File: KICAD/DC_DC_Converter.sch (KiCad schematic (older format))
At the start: 5 parts

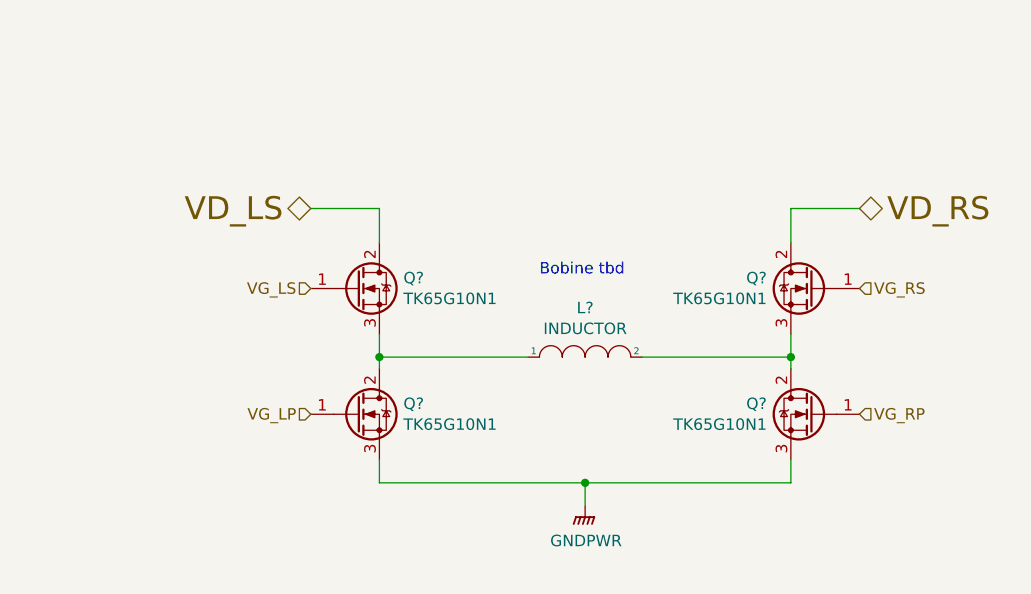
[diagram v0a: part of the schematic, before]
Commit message: ebauche driver mos
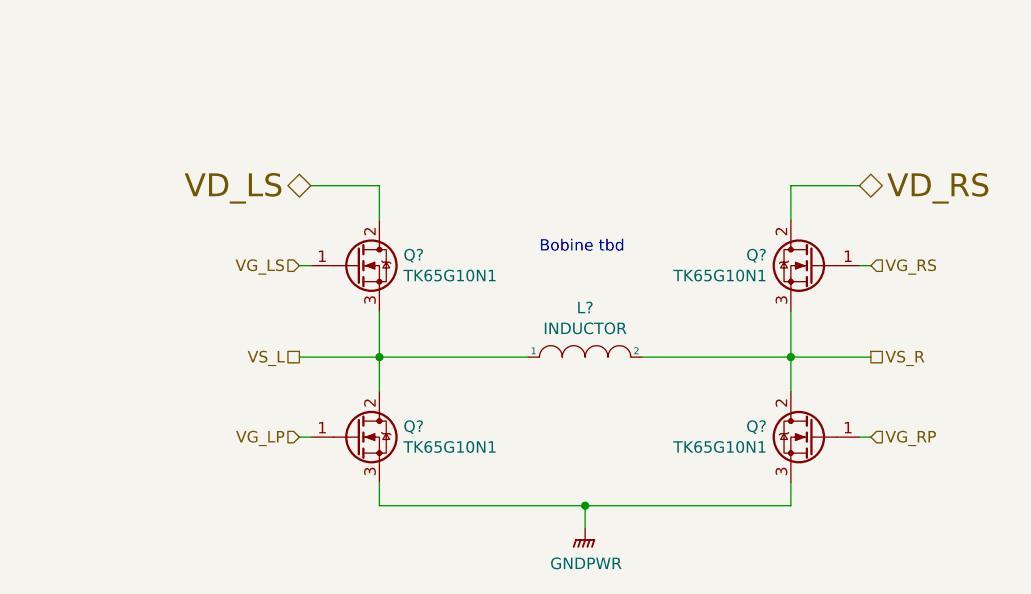
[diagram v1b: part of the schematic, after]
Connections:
- net VS_L: now reaches L?.1, Q?.2 (D), Q?.3 (S)
- net VS_R: now reaches L?.2, Q?.2 (D), Q?.3 (S)
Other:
- moved on the sheet: Q?
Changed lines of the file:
@@
 Text Notes 550  1000 0    50   ~ 0
 Entrées:\nSignaux de commande provenant du block driver permetant de controller les gates\nLes differents modes sont generer dans MOS Logic\n\nBidir:\nTension de 0 a 50v ou 5 48v TBD\n
-Text HLabel 4550 2450 0    100  BiDi ~ 0
+Text HLabel 4550 2350 0    100  BiDi ~ 0
 VD_LS
-Text HLabel 6950 2450 2    100  BiDi ~ 0
+Text HLabel 6950 2350 2    100  BiDi ~ 0
 VD_RS
-Text HLabel 4550 2800 0    50   Input ~ 0
+Text HLabel 4500 2700 0    50   Input ~ 0
 VG_LS
-Text HLabel 4550 3350 0    50   Input ~ 0
+Text HLabel 4500 3450 0    50   Input ~ 0
 VG_LP
-Text HLabel 6950 2800 2    50   Input ~ 0
+Text HLabel 7000 2700 2    50   Input ~ 0
 VG_RS
-Text HLabel 6950 3350 2    50   Input ~ 0
+Text HLabel 7000 3450 2    50   Input ~ 0
 VG_RP
 $Comp
 L Device:Q_NMOS_GDS Q?
 U 1 1 610E334F
-P 4750 2800
-F 0 "Q?" H 4955 2846 50  0000 L CNN
-F 1 "TK65G10N1" H 4955 2755 50  0000 L CNN
-F 2 "" H 4950 2900 50  0001 C CNN
-F 3 "~" H 4750 2800 50  0001 C CNN
-	1    4750 2800
+P 4750 2700
+F 0 "Q?" H 4955 2746 50  0000 L CNN
+F 1 "TK65G10N1" H 4955 2655 50  0000 L CNN
+F 2 "" H 4950 2800 50  0001 C CNN
+F 3 "~" H 4750 2700 50  0001 C CNN
+	1    4750 2700
 	1    0    0    -1
 $EndComp
@@
 L Device:Q_NMOS_GDS Q?
 U 1 1 610EEE2E
-P 4750 3350
-F 0 "Q?" H 4955 3396 50  0000 L CNN
-F 1 "TK65G10N1" H 4955 3305 50  0000 L CNN
-F 2 "" H 4950 3450 50  0001 C CNN
-F 3 "~" H 4750 3350 50  0001 C CNN
-	1    4750 3350
+P 4750 3450
+F 0 "Q?" H 4955 3496 50  0000 L CNN
+F 1 "TK65G10N1" H 4955 3405 50  0000 L CNN
+F 2 "" H 4950 3550 50  0001 C CNN
+F 3 "~" H 4750 3450 50  0001 C CNN
+	1    4750 3450
 	1    0    0    -1
 $EndComp
@@
 L Device:Q_NMOS_GDS Q?
 U 1 1 610F207F
-P 6750 2800
-F 0 "Q?" H 6955 2846 50  0000 L CNN
-F 1 "TK65G10N1" H 6955 2755 50  0000 L CNN
-F 2 "" H 6950 2900 50  0001 C CNN
-F 3 "~" H 6750 2800 50  0001 C CNN
-	1    6750 2800
+P 6750 2700
+F 0 "Q?" H 6955 2746 50  0000 L CNN
+F 1 "TK65G10N1" H 6955 2655 50  0000 L CNN
+F 2 "" H 6950 2800 50  0001 C CNN
+F 3 "~" H 6750 2700 50  0001 C CNN
+	1    6750 2700
 	-1   0    0    -1
 $EndComp
@@
 L Device:Q_NMOS_GDS Q?
 U 1 1 610F2085
-P 6750 3350
-F 0 "Q?" H 6955 3396 50  0000 L CNN
-F 1 "TK65G10N1" H 6955 3305 50  0000 L CNN
-F 2 "" H 6950 3450 50  0001 C CNN
-F 3 "~" H 6750 3350 50  0001 C CNN
-	1    6750 3350
+P 6750 3450
+F 0 "Q?" H 6955 3496 50  0000 L CNN
+F 1 "TK65G10N1" H 6955 3405 50  0000 L CNN
+F 2 "" H 6950 3550 50  0001 C CNN
+F 3 "~" H 6750 3450 50  0001 C CNN
+	1    6750 3450
 	-1   0    0    -1
 $EndComp
 Wire Wire Line
-	6650 3000 6650 3100
+	6650 2900 6650 3100
 Wire Wire Line
-	4850 3150 4850 3100
+	4850 3250 4850 3100
 Wire Wire Line
-	4850 3550 4850 3650
+	4850 3650 4850 3750
 Wire Wire Line
-	6650 3650 6650 3550
+	6650 3750 6650 3650
 $Comp
 L pspice:INDUCTOR L?
@@
 $EndComp
 Wire Wire Line
-	4850 3650 5750 3650
+	4850 3750 5750 3750
 Wire Wire Line
 	5500 3100 4850 3100
 Connection ~ 4850 3100
 Wire Wire Line
-	4850 3100 4850 3000
+	4850 3100 4850 2900
 Wire Wire Line
 	6650 3100 6000 3100
 Connection ~ 6650 3100
 Wire Wire Line
-	6650 3100 6650 3150
+	6650 3100 6650 3250
 Wire Wire Line
-	4850 2600 4850 2450
+	4850 2500 4850 2350
 Wire Wire Line
-	4550 2450 4850 2450
+	4550 2350 4850 2350
 Wire Wire Line
-	6650 2600 6650 2450
+	6650 2500 6650 2350
 Wire Wire Line
-	6950 2450 6650 2450
-Text Notes 5550 2750 0    50   ~ 0
+	6950 2350 6650 2350
+Text Notes 5550 2650 0    50   ~ 0
 Bobine tbd
 Wire Wire Line
-	5750 3750 5750 3650
-Connection ~ 5750 3650
+	5750 3850 5750 3750
+Connection ~ 5750 3750
 Wire Wire Line
-	5750 3650 6650 3650
+	5750 3750 6650 3750
 $Comp
 L power:GNDPWR #PWR?
 U 1 1 610FB372
-P 5750 3750
-F 0 "#PWR?" H 5750 3550 50  0001 C CNN
-F 1 "GNDPWR" H 5754 3596 50  0000 C CNN
-F 2 "" H 5750 3700 50  0001 C CNN
-F 3 "" H 5750 3700 50  0001 C CNN
-	1    5750 3750
+P 5750 3850
+F 0 "#PWR?" H 5750 3650 50  0001 C CNN
+F 1 "GNDPWR" H 5754 3696 50  0000 C CNN
+F 2 "" H 5750 3800 50  0001 C CNN
+F 3 "" H 5750 3800 50  0001 C CNN
+	1    5750 3850
 	1    0    0    -1
 $EndComp
+Wire Wire Line
+	7000 2700 6950 2700
+Wire Wire Line
+	7000 3450 6950 3450
+Wire Wire Line
+	4500 2700 4550 2700
+Wire Wire Line
+	4500 3450 4550 3450
+Text HLabel 4500 3100 0    50   UnSpc ~ 0
+VS_L
+Wire Wire Line
+	4500 3100 4850 3100
+Text HLabel 7000 3100 2    50   UnSpc ~ 0
+VS_R
+Wire Wire Line
+	7000 3100 6650 3100
 $EndSCHEMATC
